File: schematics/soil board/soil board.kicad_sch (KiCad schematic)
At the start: 16 parts, among them J1 AVR-ISP-6, J2 1989748, J3 1989748, J4 1989748, U1 ATtiny841-SS, U3 MCP9700Ax-ETT

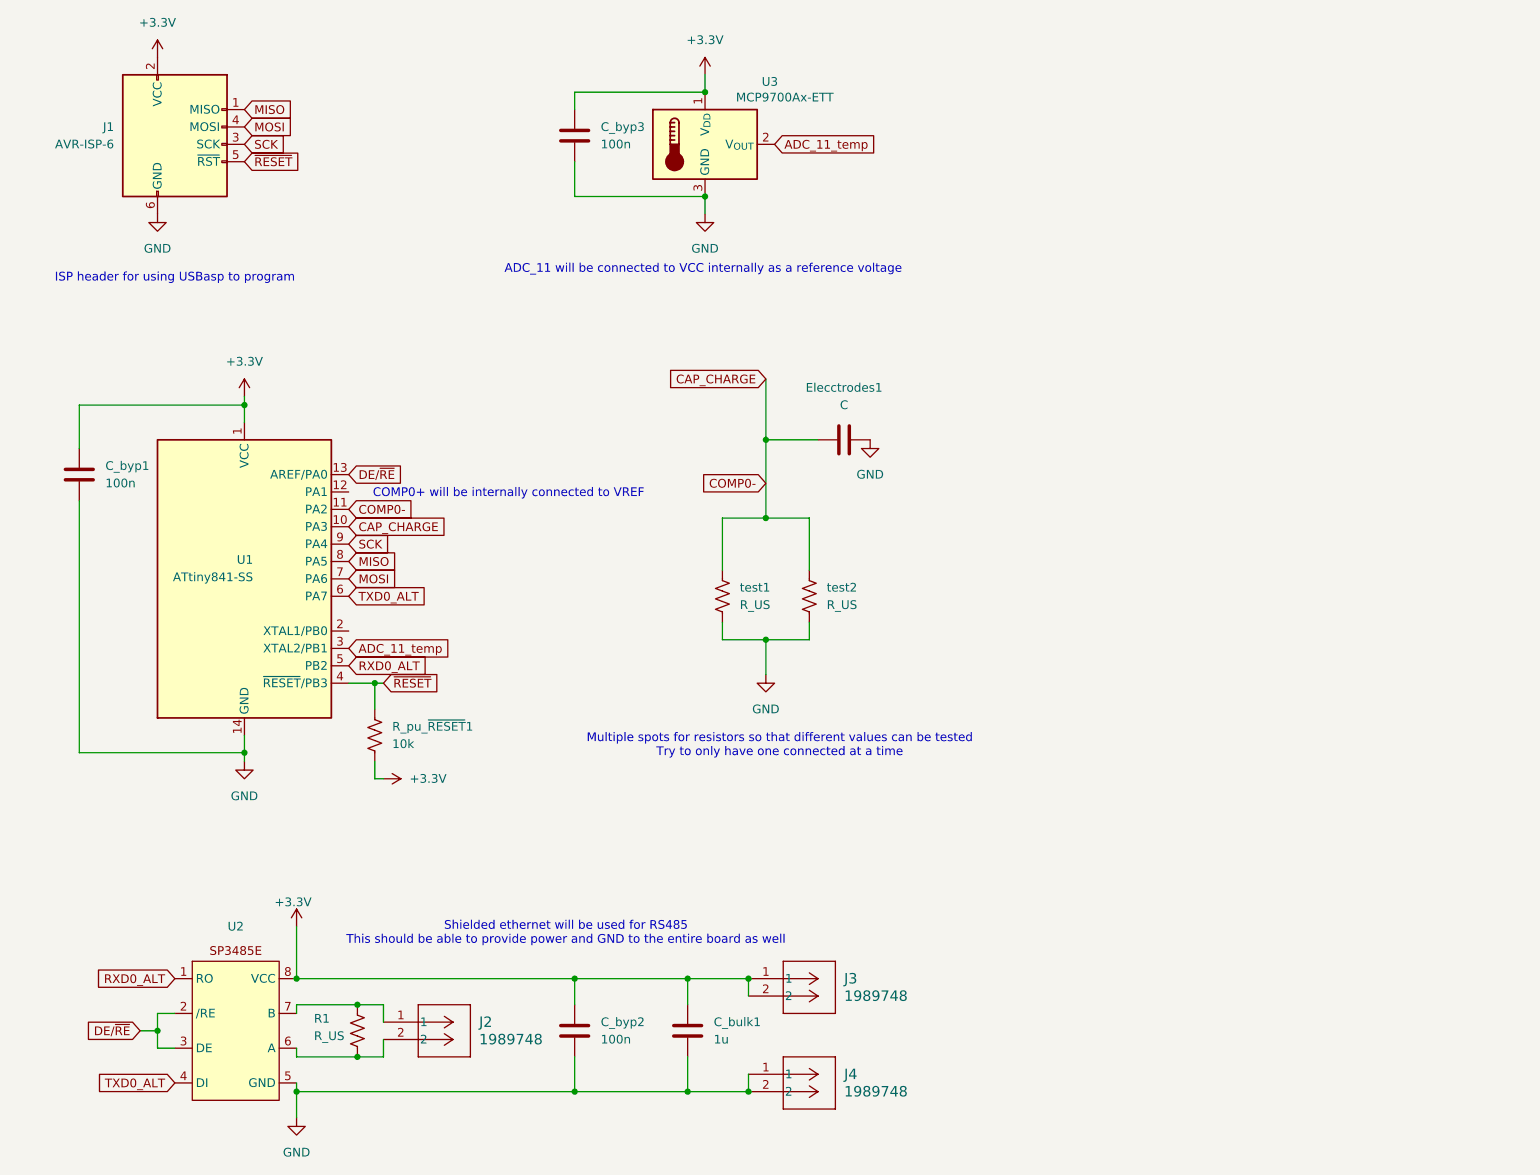
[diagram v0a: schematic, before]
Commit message: Interface for temp sensor and soil moisture sensor
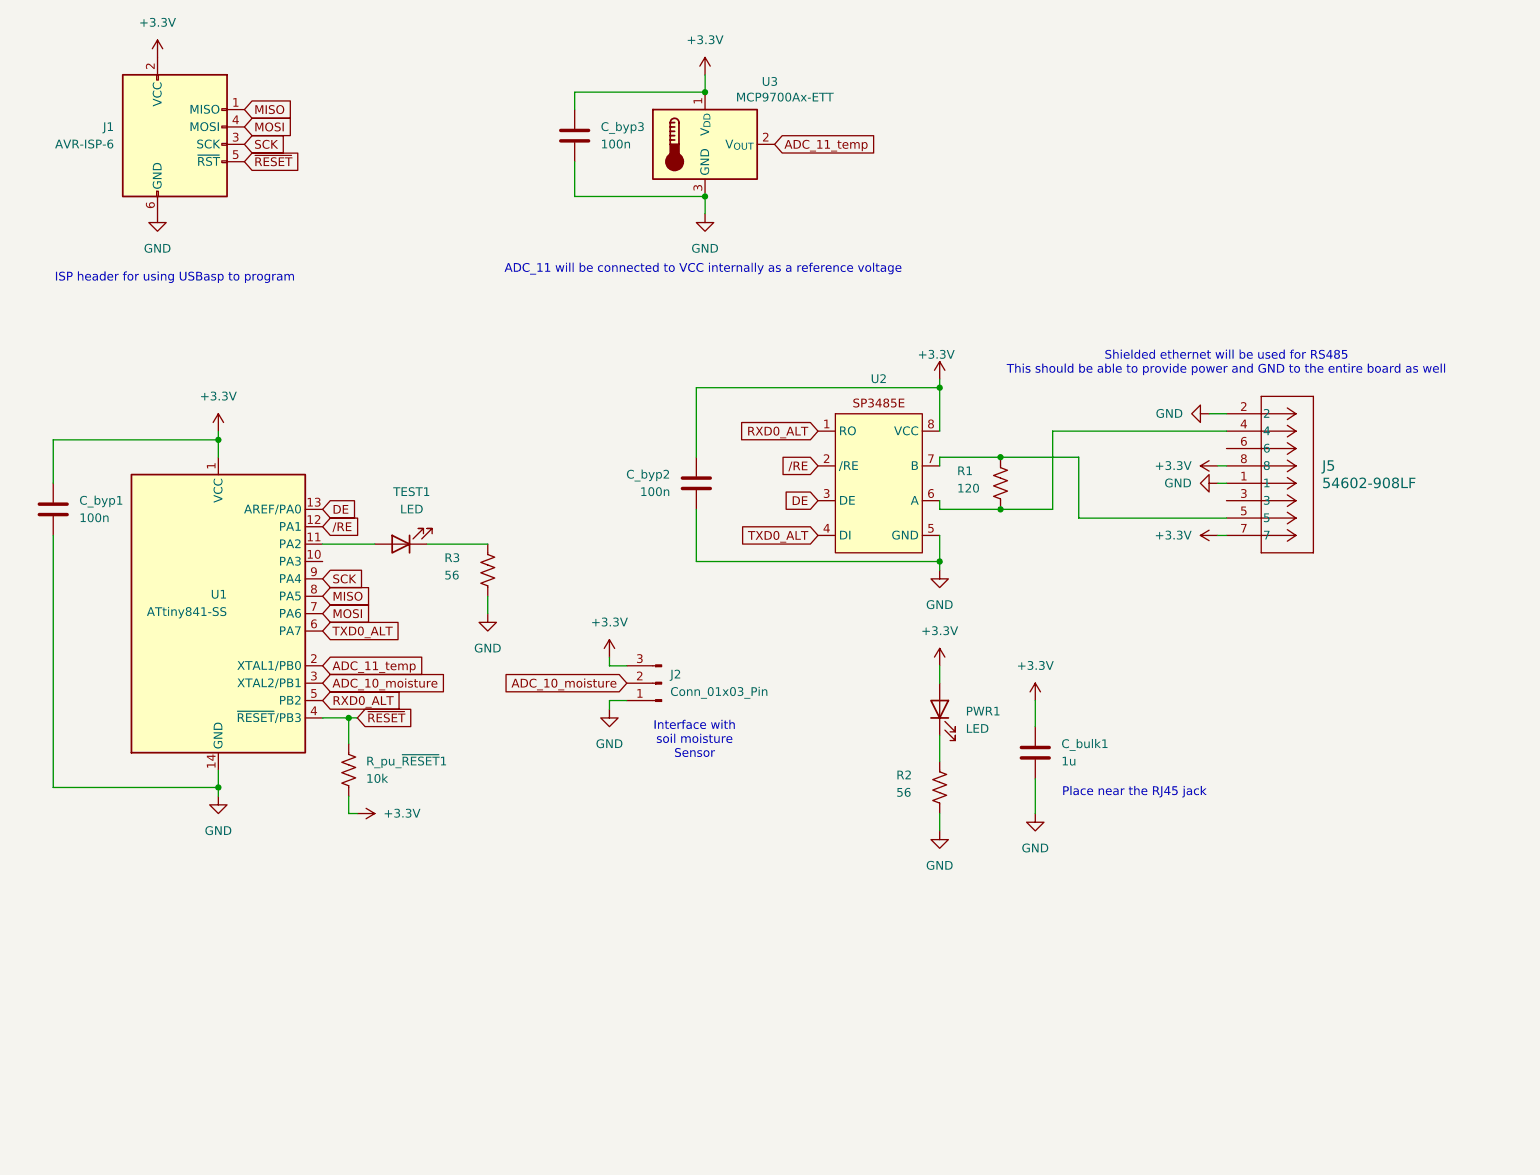
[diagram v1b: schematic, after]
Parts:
- removed Elecctrodes1: C, soil_cap:Untitled, symbol Device:C
- removed J2: 1989748, footprints:CONN_1989748_PXC, symbol 2026-10-16_21-18-38:1989748
- removed J3, J4: 1989748, CONN_1989748_PXC, symbol 2026-10-16_21-18-38:1989748
- removed test1, test2: R_US, Resistor_THT:R_Axial_DIN0207_L6.3mm_D2.5mm_P7.62mm_Horizontal, symbol Device:R_US
- added J2: Conn_01x03_Pin, Connector_PinHeader_2.54mm:PinHeader_1x03_P2.54mm_Vertical, symbol Connector:Conn_01x03_Pin
- added J5: 54602-908LF, CONN8_2-908LF_AMP, symbol 2026-10-21_23-02-14:54602-908LF
- added PWR1, TEST1: LED, LED_SMD:LED_0805_2012Metric_Pad1.15x1.40mm_HandSolder, symbol Device:LED
- added R2, R3: 56, Resistor_SMD:R_0805_2012Metric_Pad1.20x1.40mm_HandSolder, symbol Device:R_US
- R1: value R_US -> 120
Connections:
- net +3.3V: now also J2.3 (Pin_3), J5.7, J5.8, PWR1.2 (A)
- net ADC_11_temp: now also U1.2 (XTAL1/PB0); no longer U1.3 (XTAL2/PB1)
- net GND: now also J2.1 (Pin_1), J5.1, J5.2, R2.2, R3.2
- net /RE: now reaches U1.12 (PA1)
- net /RE: now also U2.2 (/RE)
- net at R1.2, U2.6 (A): now also J5.4
- net at R1.1, U2.7 (B): now also J5.5
- net CAP_CHARGE: no longer names the net of U1.11 (PA2)
- net CAP_CHARGE: now also TEST1.2 (A); no longer U1.10 (PA3)
- net DE/~{RE} renamed DE
- net DE: no longer U2.2 (/RE)
- new net: PWR1.1 (K), R2.1
- new net: R3.1, TEST1.1 (K)
- new net ADC_10_moisture: J2.2 (Pin_2), U1.3 (XTAL2/PB1)
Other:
- note added: "Interface with soil moisture Sensor"
- note added: "Place near the RJ45 jack"
- note removed: "COMP0+ will be internally connected to VREF"
- note removed: "Multiple spots for resistors so that different values can be tested Try to only have one connected at a time"
- moved on the sheet: C_bulk1, C_byp1, C_byp2, R1, R_pu_~{RESET}1, U1, U2
